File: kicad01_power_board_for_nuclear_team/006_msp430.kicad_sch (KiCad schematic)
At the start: 6 parts

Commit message: ix
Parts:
- R603: symbol 01dyn_lib:R0805_0.0 -> 1001_un:R0805_0.0
- R604: footprint Resistor_SMD:R_0603_1608Metric_Pad0.98x0.95mm_HandSolder -> 02_dyn_pcblib:C0603; symbol 01dyn_lib:R0603_DNP -> 1001_un:R0603_DNP
- R623, R624, R633, R634: footprint Resistor_SMD:R_0603_1608Metric -> 02_dyn_pcblib:C0603; symbol 01dyn_lib:R0603_10k -> 1001_un:R0603_10k
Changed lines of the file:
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@@
     )
   )
-  (symbol (lib_id "01dyn_lib:R0805_0.0") (at 73.66 54.61 0) (unit 1)
+  (symbol (lib_id "1001_un:R0805_0.0") (at 73.66 54.61 0) (unit 1)
     (in_bom yes) (on_board yes) (fields_autoplaced)
     (property "Reference" "R603" (id 0) (at 73.66 49.53 0)
@@
     (pin "2")
   )
-  (symbol (lib_id "01dyn_lib:R0603_10k") (at 105.41 63.5 0) (unit 1)
+  (symbol (lib_id "1001_un:R0603_10k") (at 105.41 63.5 0) (unit 1)
     (in_bom yes) (on_board yes) (fields_autoplaced)
     (property "Reference" "R624" (id 0) (at 105.41 58.42 0)
@@
       (effects (font (size 0.5 0.5)))
     )
-    (property "Footprint" "Resistor_SMD:R_0603_1608Metric" (id 2) (at 106.68 59.69 0)
+    (property "Footprint" "02_dyn_pcblib:C0603" (id 2) (at 106.68 59.69 0)
       (effects (font (size 1.27 1.27)) hide)
     )
@@
     (pin "2")
   )
-  (symbol (lib_name "R0603_10k_2") (lib_id "01dyn_lib:R0603_10k") (at 73.66 63.5 0) (unit 1)
+  (symbol (lib_id "1001_un:R0603_10k") (at 73.66 63.5 0) (unit 1)
     (in_bom yes) (on_board yes) (fields_autoplaced)
     (property "Reference" "R623" (id 0) (at 73.66 58.42 0)
@@
       (effects (font (size 0.5 0.5)))
     )
-    (property "Footprint" "Resistor_SMD:R_0603_1608Metric" (id 2) (at 74.93 59.69 0)
+    (property "Footprint" "02_dyn_pcblib:C0603" (id 2) (at 74.93 59.69 0)
       (effects (font (size 1.27 1.27)) hide)
     )
@@
     (pin "2")
   )
-  (symbol (lib_id "01dyn_lib:R0603_DNP") (at 105.41 54.61 0) (unit 1)
+  (symbol (lib_id "1001_un:R0603_DNP") (at 105.41 54.61 0) (unit 1)
     (in_bom yes) (on_board yes) (fields_autoplaced)
     (property "Reference" "R604" (id 0) (at 105.41 49.53 0)
@@
       (effects (font (size 0.5 0.5)) hide)
     )
-    (property "Footprint" "Resistor_SMD:R_0603_1608Metric_Pad0.98x0.95mm_HandSolder" (id 2) (at 106.68 50.8 0)
+    (property "Footprint" "02_dyn_pcblib:C0603" (id 2) (at 106.68 50.8 0)
       (effects (font (size 1.27 1.27)) hide)
     )
@@
     (pin "2")
   )
-  (symbol (lib_name "R0603_10k_3") (lib_id "01dyn_lib:R0603_10k") (at 73.66 72.39 0) (unit 1)
+  (symbol (lib_id "1001_un:R0603_10k") (at 73.66 72.39 0) (unit 1)
     (in_bom yes) (on_board yes) (fields_autoplaced)
     (property "Reference" "R633" (id 0) (at 73.66 67.31 0)
@@
       (effects (font (size 0.5 0.5)))
     )
-    (property "Footprint" "Resistor_SMD:R_0603_1608Metric" (id 2) (at 74.93 68.58 0)
+    (property "Footprint" "02_dyn_pcblib:C0603" (id 2) (at 74.93 68.58 0)
       (effects (font (size 1.27 1.27)) hide)
     )
@@
     (pin "2")
   )
-  (symbol (lib_name "R0603_10k_1") (lib_id "01dyn_lib:R0603_10k") (at 105.41 72.39 0) (unit 1)
+  (symbol (lib_id "1001_un:R0603_10k") (at 105.41 72.39 0) (unit 1)
     (in_bom yes) (on_board yes) (fields_autoplaced)
     (property "Reference" "R634" (id 0) (at 105.41 67.31 0)
@@
       (effects (font (size 0.5 0.5)))
     )
-    (property "Footprint" "Resistor_SMD:R_0603_1608Metric" (id 2) (at 106.68 68.58 0)
+    (property "Footprint" "02_dyn_pcblib:C0603" (id 2) (at 106.68 68.58 0)
       (effects (font (size 1.27 1.27)) hide)
     )

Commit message: x
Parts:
- R603: symbol 1001_un:R0805_0.0 -> 1002_res:R0805_0.0
- R604: symbol 1001_un:R0603_DNP -> 1002_res:R0603_DNP
- R623, R624, R633, R634: symbol 1001_un:R0603_10k -> 1002_res:R0603_10k
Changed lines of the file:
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@@
     )
   )
-  (symbol (lib_id "1001_un:R0805_0.0") (at 73.66 54.61 0) (unit 1)
+  (symbol (lib_id "1002_res:R0805_0.0") (at 73.66 54.61 0) (unit 1)
     (in_bom yes) (on_board yes) (fields_autoplaced)
     (property "Reference" "R603" (id 0) (at 73.66 49.53 0)
@@
     (pin "2")
   )
-  (symbol (lib_id "1001_un:R0603_10k") (at 105.41 63.5 0) (unit 1)
+  (symbol (lib_id "1002_res:R0603_10k") (at 105.41 63.5 0) (unit 1)
     (in_bom yes) (on_board yes) (fields_autoplaced)
     (property "Reference" "R624" (id 0) (at 105.41 58.42 0)
@@
     (pin "2")
   )
-  (symbol (lib_id "1001_un:R0603_10k") (at 73.66 63.5 0) (unit 1)
+  (symbol (lib_id "1002_res:R0603_10k") (at 73.66 63.5 0) (unit 1)
     (in_bom yes) (on_board yes) (fields_autoplaced)
     (property "Reference" "R623" (id 0) (at 73.66 58.42 0)
@@
     (pin "2")
   )
-  (symbol (lib_id "1001_un:R0603_DNP") (at 105.41 54.61 0) (unit 1)
+  (symbol (lib_id "1002_res:R0603_DNP") (at 105.41 54.61 0) (unit 1)
     (in_bom yes) (on_board yes) (fields_autoplaced)
     (property "Reference" "R604" (id 0) (at 105.41 49.53 0)
@@
     (pin "2")
   )
-  (symbol (lib_id "1001_un:R0603_10k") (at 73.66 72.39 0) (unit 1)
+  (symbol (lib_id "1002_res:R0603_10k") (at 73.66 72.39 0) (unit 1)
     (in_bom yes) (on_board yes) (fields_autoplaced)
     (property "Reference" "R633" (id 0) (at 73.66 67.31 0)
@@
     (pin "2")
   )
-  (symbol (lib_id "1001_un:R0603_10k") (at 105.41 72.39 0) (unit 1)
+  (symbol (lib_id "1002_res:R0603_10k") (at 105.41 72.39 0) (unit 1)
     (in_bom yes) (on_board yes) (fields_autoplaced)
     (property "Reference" "R634" (id 0) (at 105.41 67.31 0)

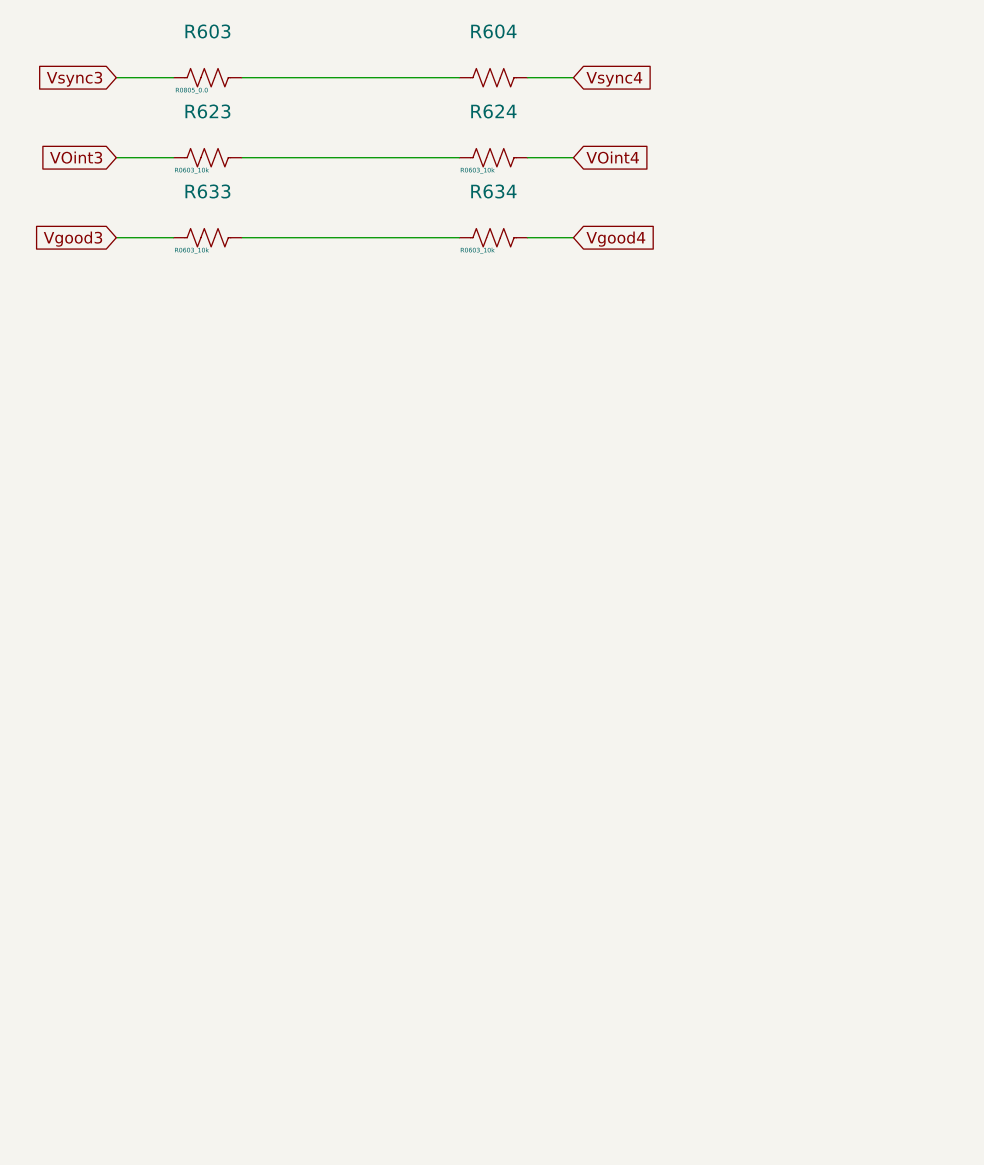
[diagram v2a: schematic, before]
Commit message: x
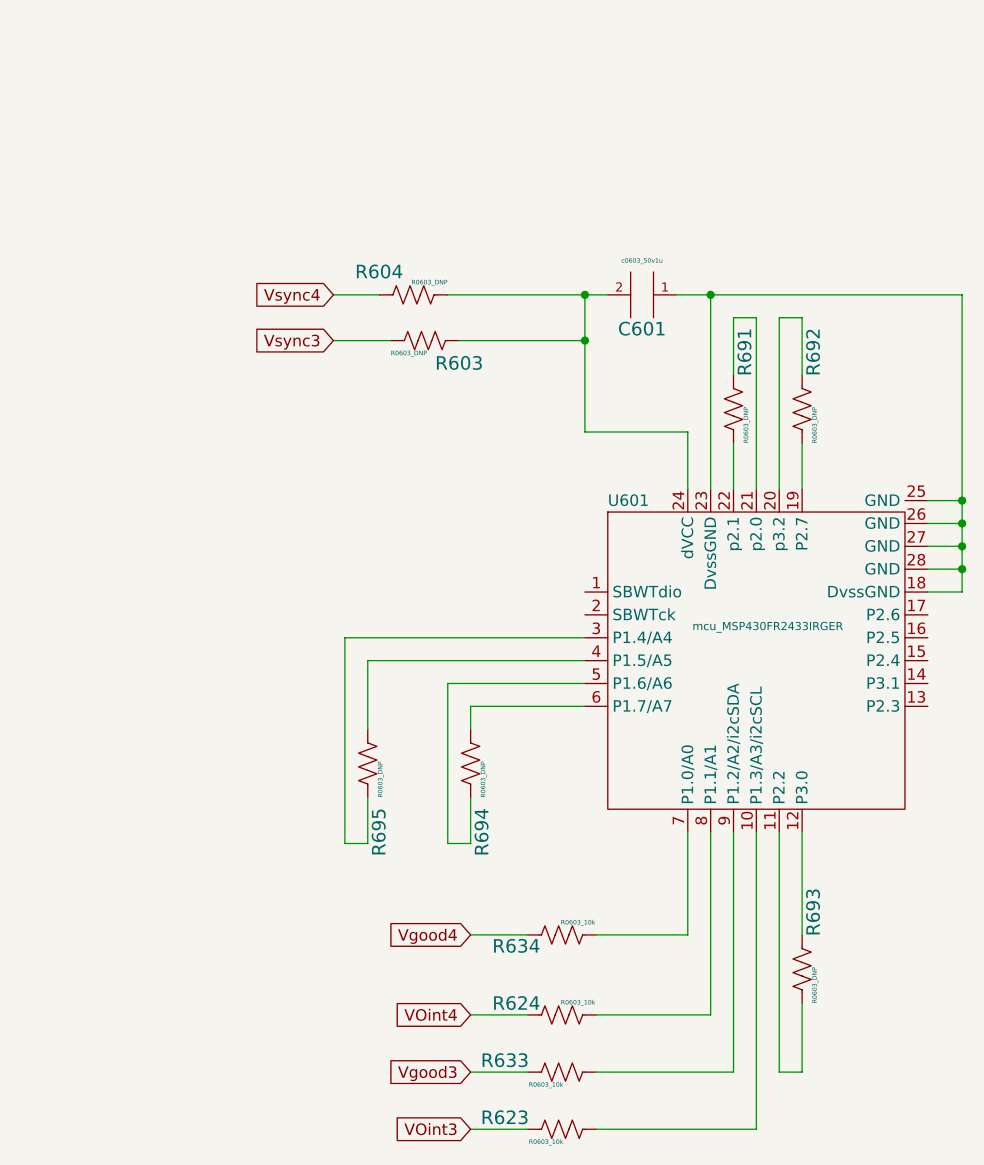
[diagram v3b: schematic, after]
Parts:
- added C601: c0603_50v1u, 02_dyn_pcblib:C0603, symbol 1003_cap:c0603_50v1u
- added R691, R692, R693, R694, R695: R0603_DNP, 02_dyn_pcblib:C0603, symbol 1002_res:R0603_DNP
- added U601: mcu_MSP430FR2433IRGER, 02_dyn_pcblib:QFN-24-1EP_4x4mm_P0.5mm_EP2.8x2.8mmX, symbol 1009_ic:mcu_MSP430FR2433IRGER
- R603: value R0805_0.0 -> R0603_DNP; footprint 02_dyn_pcblib:R0805mix0603 -> 02_dyn_pcblib:C0603; symbol 1002_res:R0805_0.0 -> 1002_res:R0603_DNP; Notice (none) -> This DNP resistor use handly footprint, which is larger tha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; PartDesc 0 Ohms Jumper 0.125W, 1/8W Chip Resistor 0805 (2012 Metric)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 -> (none); PartNum RC0805JR-070RL -> R0603_DNP
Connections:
- net at R603.2, R604.1: now also C601.2, U601.24 (dVCC)
- net at R623.2: now also U601.10 (P1.3/A3/i2cSCL); no longer R624.1
- net at R634.1: now also U601.7 (P1.0/A0); no longer R633.2
- new net: C601.1, U601.18 (DvssGND), U601.23 (DvssGND), U601.25 (GND), U601.26 (GND), U601.27 (GND), U601.28 (GND)
- new net: R693.1, U601.11 (P2.2)
- new net: R693.2, U601.12 (P3.0)
- new net: R692.1, U601.19 (P2.7)
- new net: R692.2, U601.20 (p3.2)
- new net: R691.2, U601.21 (p2.0)
- new net: R691.1, U601.22 (p2.1)
- new net: R695.1, U601.3 (P1.4/A4)
- new net: R695.2, U601.4 (P1.5/A5)
- new net: R694.1, U601.5 (P1.6/A6)
- new net: R694.2, U601.6 (P1.7/A7)
- new net: R624.1, U601.8 (P1.1/A1)
- new net: R633.2, U601.9 (P1.2/A2/i2cSDA)
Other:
- moved on the sheet: R603, R604, R623, R624, R633, R634
